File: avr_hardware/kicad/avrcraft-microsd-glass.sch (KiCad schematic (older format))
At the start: 61 parts, among them J1 AVRISP6, J2 MICROSD_1050270001, P1 ETHERNET, P10 CONN_1, P11 CONN_1, P2 CONN_1, P3 CONN_1, P4 CONN_1, P5 CONN_1, P6 CONN_1, P7 CONN_1, P8 CONN_7, P9 CONN_1, T1 S553-5999-52, U1 ATMEGA328, U2 MCP1824, U3 ENC424J600, U4 MCP1824, U5 OPA832, X1 XTAL4P, X2 25MHz

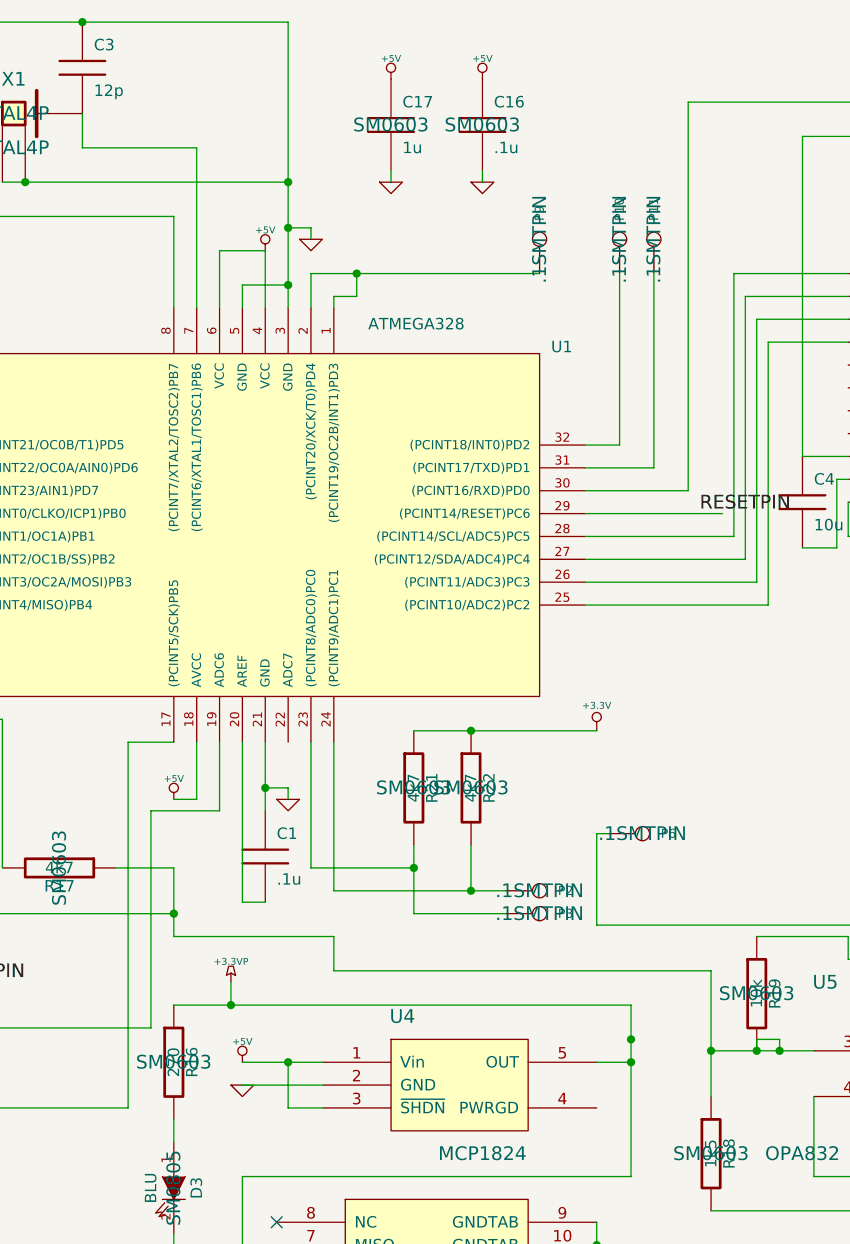
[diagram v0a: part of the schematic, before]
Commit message: update all the boards ! yay.
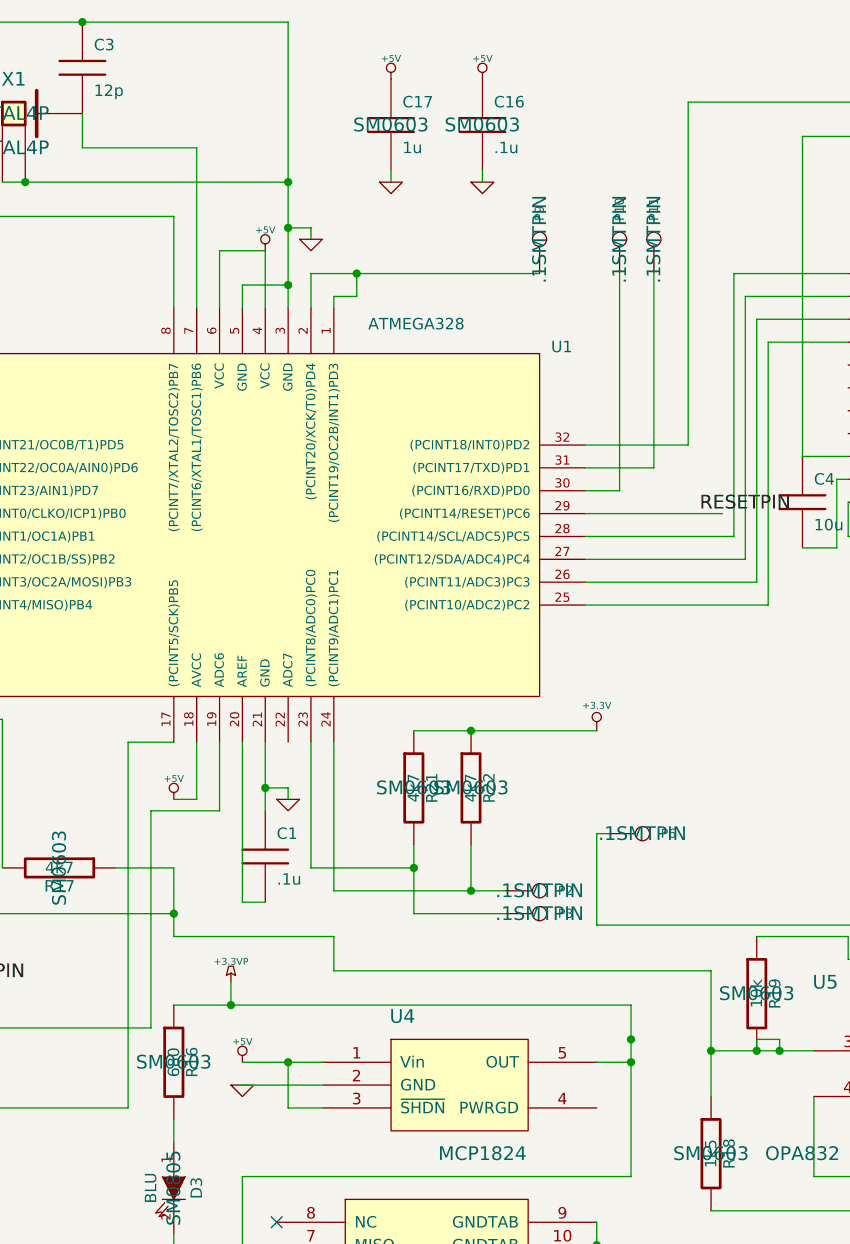
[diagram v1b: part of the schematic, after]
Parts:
- R16: value 270 -> 680
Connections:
- net at R4.2, U3.24 (~INT~/SPISEL): now also U1.32 ((PCINT18/INT0)PD2); no longer U1.30 ((PCINT16/RXD)PD0)
- net at P10.1: now also U1.30 ((PCINT16/RXD)PD0); no longer U1.32 ((PCINT18/INT0)PD2)
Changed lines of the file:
@@
-EESchema Schematic File Version 2  date Tue 12 Feb 2013 09:33:11 PM EST
+EESchema Schematic File Version 2  date Wed 13 Feb 2013 10:58:59 AM EST
 LIBS:power
 LIBS:device
@@
 Comment4 ""
 $EndDescr
+Wire Wire Line
+	5350 2350 5350 850
+Wire Wire Line
+	5350 2350 4900 2350
 Connection ~ 3900 1600
 Wire Wire Line
 	4700 1600 3700 1600
-Wire Wire Line
-	5050 1600 5050 2350
-Wire Wire Line
-	5050 2350 4900 2350
-Wire Wire Line
-	4900 2550 5350 2550
-Wire Wire Line
-	5350 2550 5350 850
 Wire Wire Line
 	5350 850  7550 850
@@
 Wire Wire Line
 	3900 1700 3900 1600
+Wire Wire Line
+	5050 1600 5050 2550
+Wire Wire Line
+	5050 2550 4900 2550
 $Comp
 L CONN_1 P9
@@
 P 3100 5050
 F 0 "R16" V 3180 5050 50  0000 C CNN
-F 1 "270" V 3100 5050 50  0000 C CNN
+F 1 "680" V 3100 5050 50  0000 C CNN
 F 2 "SM0603" H 3100 5050 60  0000 C CNN
 	1    3100 5050
